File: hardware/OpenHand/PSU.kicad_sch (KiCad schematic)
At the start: 0 parts

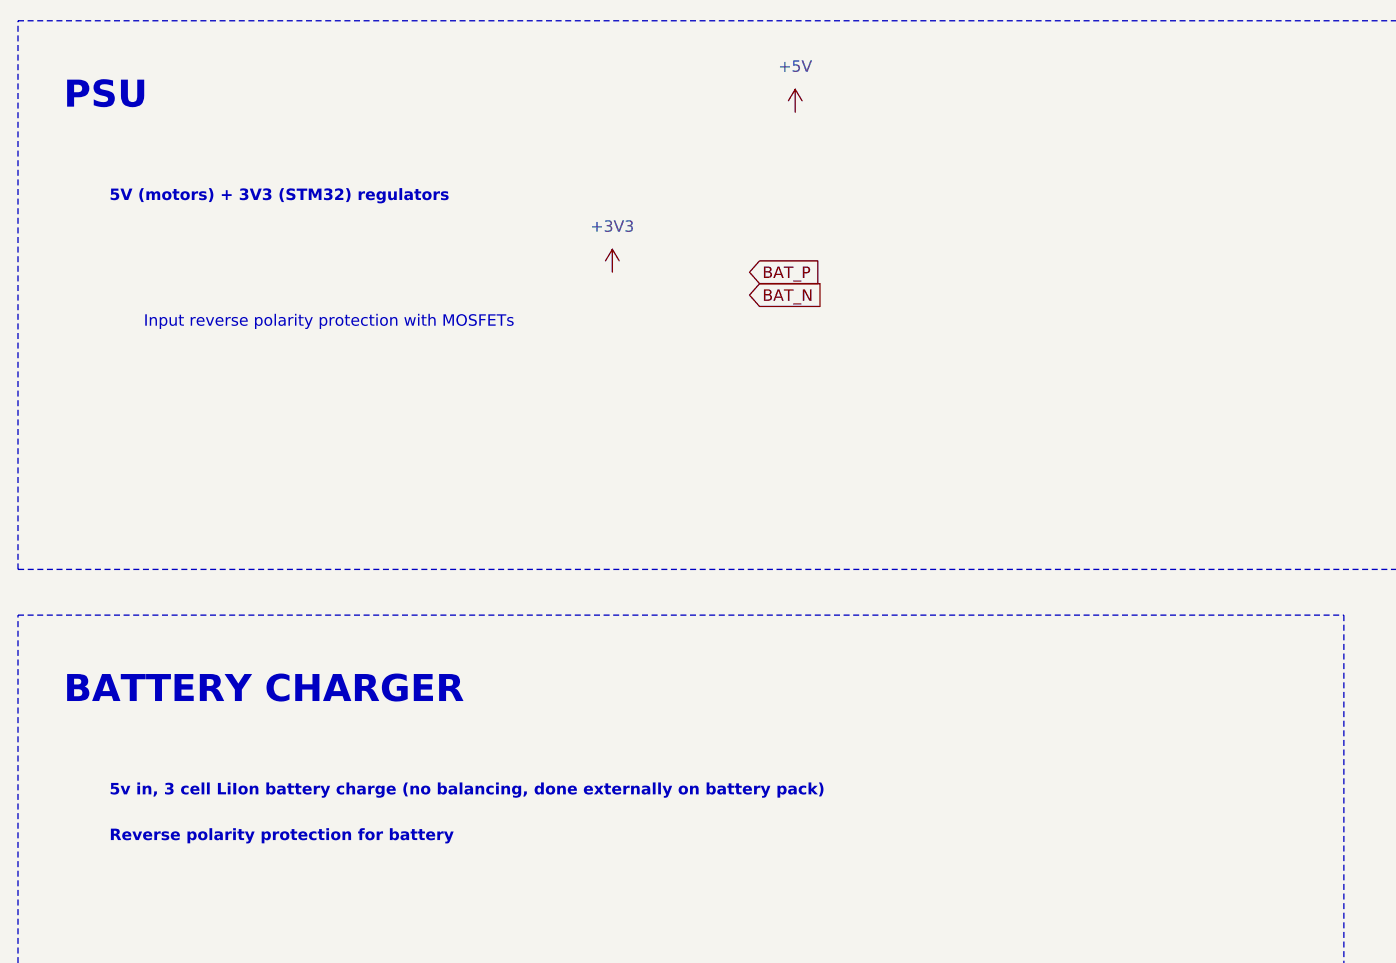
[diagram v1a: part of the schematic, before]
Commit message: Update schematic a bit
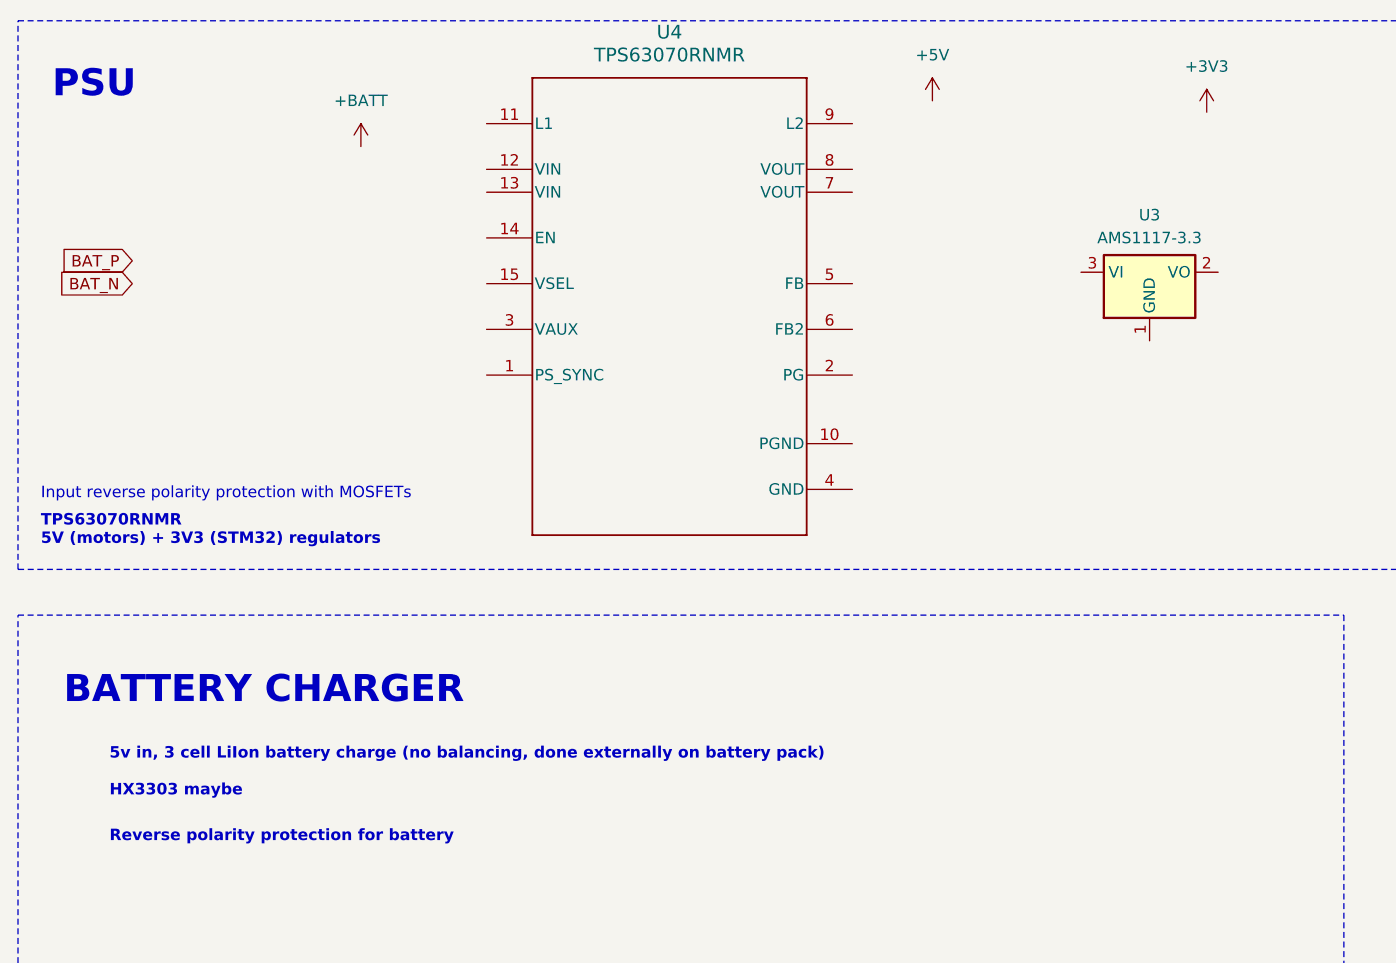
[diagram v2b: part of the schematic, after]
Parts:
- added U3: AMS1117-3.3, Package_TO_SOT_SMD:SOT-223-3_TabPin2, symbol Regulator_Linear:AMS1117-3.3
- added U4: TPS63070RNMR, symbol TPS63070RNMR:TPS63070RNMR
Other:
- note added: "5v in, 3 cell LiIon battery charge (no balancing, done externally on battery pack) HX3303 maybe"
- note added: "TPS63070RNMR 5V (motors) + 3V3 (STM32) regulators"
- note removed: "5V (motors) + 3V3 (STM32) regulators"
- note removed: "5v in, 3 cell LiIon battery charge (no balancing, done externally on battery pack)"
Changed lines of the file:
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@@
     (fill (type none))
   )
-  (text "5v in, 3 cell LiIon battery charge (no balancing, done externally on battery pack)"
+  (text "5v in, 3 cell LiIon battery charge (no balancing, done externally on battery pack)\n\nHX3303 maybe"
     (at 33.02 109.22 0)
     (effects (font (size 1.27 1.27) bold) (justify left bottom))
   )
-  (text "Input reverse polarity protection with MOSFETs" (at 36.83 57.15 0)
+  (text "Input reverse polarity protection with MOSFETs" (at 25.4 76.2 0)
     (effects (font (size 1.27 1.27)) (justify left bottom))
   )
@@
     (effects (font (size 1.27 1.27) bold) (justify left bottom))
   )
-  (text "PSU" (at 27.94 33.02 0)
+  (text "PSU" (at 26.67 31.75 0)
     (effects (font (size 3 3) (thickness 0.6) bold) (justify left bottom))
   )
@@
     (effects (font (size 3 3) (thickness 0.6) bold) (justify left bottom))
   )
-  (text "5V (motors) + 3V3 (STM32) regulators" (at 33.02 43.18 0)
+  (text "TPS63070RNMR \n5V (motors) + 3V3 (STM32) regulators"
+    (at 25.4 81.28 0)
     (effects (font (size 1.27 1.27) bold) (justify left bottom))
   )
-  (global_label "BAT_N" (shape input) (at 104.14 53.34 0) (fields_autoplaced)
-    (effects (font (size 1.27 1.27)) (justify left))
-    (property "Intersheetrefs" "${INTERSHEET_REFS}" (at 112.7495 53.34 0)
-      (effects (font (size 1.27 1.27)) (justify left) hide)
+  (global_label "BAT_N" (shape input) (at 35.56 52.07 180) (fields_autoplaced)
+    (effects (font (size 1.27 1.27)) (justify right))
+    (property "Intersheetrefs" "${INTERSHEET_REFS}" (at 26.9505 52.07 0)
+      (effects (font (size 1.27 1.27)) (justify right) hide)
     )
   )
-  (global_label "BAT_P" (shape input) (at 104.14 50.8 0) (fields_autoplaced)
-    (effects (font (size 1.27 1.27)) (justify left))
-    (property "Intersheetrefs" "${INTERSHEET_REFS}" (at 112.689 50.8 0)
-      (effects (font (size 1.27 1.27)) (justify left) hide)
+  (global_label "BAT_P" (shape input) (at 35.56 49.53 180) (fields_autoplaced)
+    (effects (font (size 1.27 1.27)) (justify right))
+    (property "Intersheetrefs" "${INTERSHEET_REFS}" (at 27.011 49.53 0)
+      (effects (font (size 1.27 1.27)) (justify right) hide)
     )
   )
-  (symbol (lib_id "power:+5V") (at 109.22 33.02 0) (unit 1)
+  (symbol (lib_id "Regulator_Linear:AMS1117-3.3") (at 148.59 50.8 0) (unit 1)
     (in_bom yes) (on_board yes) (dnp no) (fields_autoplaced)
-    (property "Reference" "#PWR01" (at 109.22 36.83 0)
+    (property "Reference" "U3" (at 148.59 44.45 0)
+      (effects (font (size 1.27 1.27)))
+    )
+    (property "Value" "AMS1117-3.3" (at 148.59 46.99 0)
+      (effects (font (size 1.27 1.27)))
+    )
+    (property "Footprint" "Package_TO_SOT_SMD:SOT-223-3_TabPin2" (at 148.59 45.72 0)
       (effects (font (size 1.27 1.27)) hide)
     )
-    (property "Value" "+5V" (at 109.22 27.94 0)
+    (property "Datasheet" "http://www.advanced-monolithic.com/pdf/ds1117.pdf" (at 151.13 57.15 0)
+      (effects (font (size 1.27 1.27)) hide)
+    )
+    (pin "1")
+    (pin "2")
+    (pin "3")
+    (instances
+      (project "OpenHand"
+        (path "/f1fbd835-8408-4592-854c-2fbec9d052ec/11b37193-b902-4bf9-977f-96c37af6f134"
+          (reference "U3") (unit 1)
+        )
+      )
+    )
+  )
+  (symbol (lib_id "power:+BATT") (at 60.96 36.83 0) (unit 1)
+    (in_bom yes) (on_board yes) (dnp no) (fields_autoplaced)
+    (property "Reference" "#PWR036" (at 60.96 40.64 0)
+      (effects (font (size 1.27 1.27)) hide)
+    )
+    (property "Value" "+BATT" (at 60.96 31.75 0)
       (effects (font (size 1.27 1.27)))
     )
-    (property "Footprint" "" (at 109.22 33.02 0)
+    (property "Footprint" "" (at 60.96 36.83 0)
       (effects (font (size 1.27 1.27)) hide)
     )
-    (property "Datasheet" "" (at 109.22 33.02 0)
+    (property "Datasheet" "" (at 60.96 36.83 0)
+      (effects (font (size 1.27 1.27)) hide)
+    )
+    (pin "1")
+    (instances
+      (project "OpenHand"
+        (path "/f1fbd835-8408-4592-854c-2fbec9d052ec/11b37193-b902-4bf9-977f-96c37af6f134"
+          (reference "#PWR036") (unit 1)
+        )
+      )
+    )
+  )
+  (symbol (lib_id "power:+5V") (at 124.46 31.75 0) (unit 1)
+    (in_bom yes) (on_board yes) (dnp no) (fields_autoplaced)
+    (property "Reference" "#PWR01" (at 124.46 35.56 0)
+      (effects (font (size 1.27 1.27)) hide)
+    )
+    (property "Value" "+5V" (at 124.46 26.67 0)
+      (effects (font (size 1.27 1.27)))
+    )
+    (property "Footprint" "" (at 124.46 31.75 0)
+      (effects (font (size 1.27 1.27)) hide)
+    )
+    (property "Datasheet" "" (at 124.46 31.75 0)
       (effects (font (size 1.27 1.27)) hide)
     )
@@
     )
   )
-  (symbol (lib_id "power:+3V3") (at 88.9 50.8 0) (unit 1)
+  (symbol (lib_id "TPS63070RNMR:TPS63070RNMR") (at 95.25 54.61 0) (unit 1)
     (in_bom yes) (on_board yes) (dnp no) (fields_autoplaced)
-    (property "Reference" "#PWR040" (at 88.9 54.61 0)
+    (property "Reference" "U4" (at 95.25 24.13 0)
+      (effects (font (size 1.524 1.524)))
+    )
+    (property "Value" "TPS63070RNMR" (at 95.25 26.67 0)
+      (effects (font (size 1.524 1.524)))
+    )
+    (property "Footprint" "" (at 95.25 54.61 0)
+      (effects (font (size 1.27 1.27) italic) hide)
+    )
+    (property "Datasheet" "TPS63070RNMR" (at 95.25 54.61 0)
+      (effects (font (size 1.27 1.27) italic) hide)
+    )
+    (pin "1")
+    (pin "10")
+    (pin "11")
+    (pin "12")
+    (pin "13")
+    (pin "14")
+    (pin "15")
+    (pin "2")
+    (pin "3")
+    (pin "4")
+    (pin "5")
+    (pin "6")
+    (pin "7")
+    (pin "8")
+    (pin "9")
+    (instances
+      (project "OpenHand"
+        (path "/f1fbd835-8408-4592-854c-2fbec9d052ec/11b37193-b902-4bf9-977f-96c37af6f134"
+          (reference "U4") (unit 1)
+        )
+      )
+    )
+  )
+  (symbol (lib_id "power:+3V3") (at 154.94 33.02 0) (unit 1)
+    (in_bom yes) (on_board yes) (dnp no) (fields_autoplaced)
+    (property "Reference" "#PWR040" (at 154.94 36.83 0)
       (effects (font (size 1.27 1.27)) hide)
     )
-    (property "Value" "+3V3" (at 88.9 45.72 0)
+    (property "Value" "+3V3" (at 154.94 27.94 0)
       (effects (font (size 1.27 1.27)))
     )
-    (property "Footprint" "" (at 88.9 50.8 0)
+    (property "Footprint" "" (at 154.94 33.02 0)
       (effects (font (size 1.27 1.27)) hide)
     )
-    (property "Datasheet" "" (at 88.9 50.8 0)
+    (property "Datasheet" "" (at 154.94 33.02 0)
       (effects (font (size 1.27 1.27)) hide)
     )

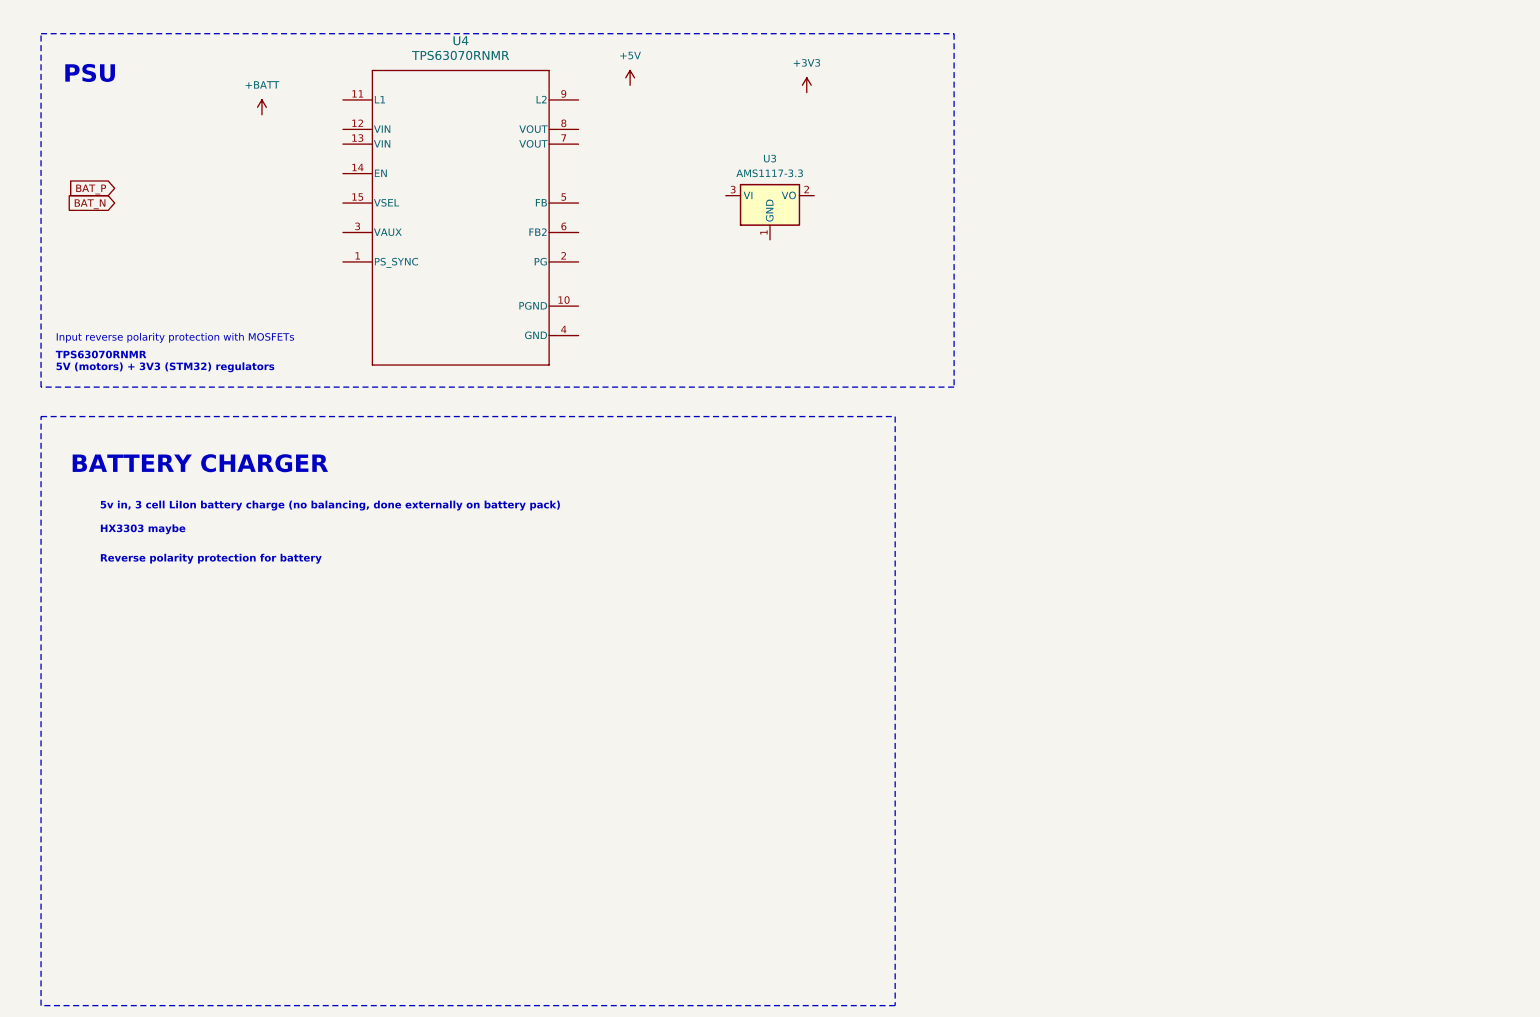
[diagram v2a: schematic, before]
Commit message: Update sch and board design
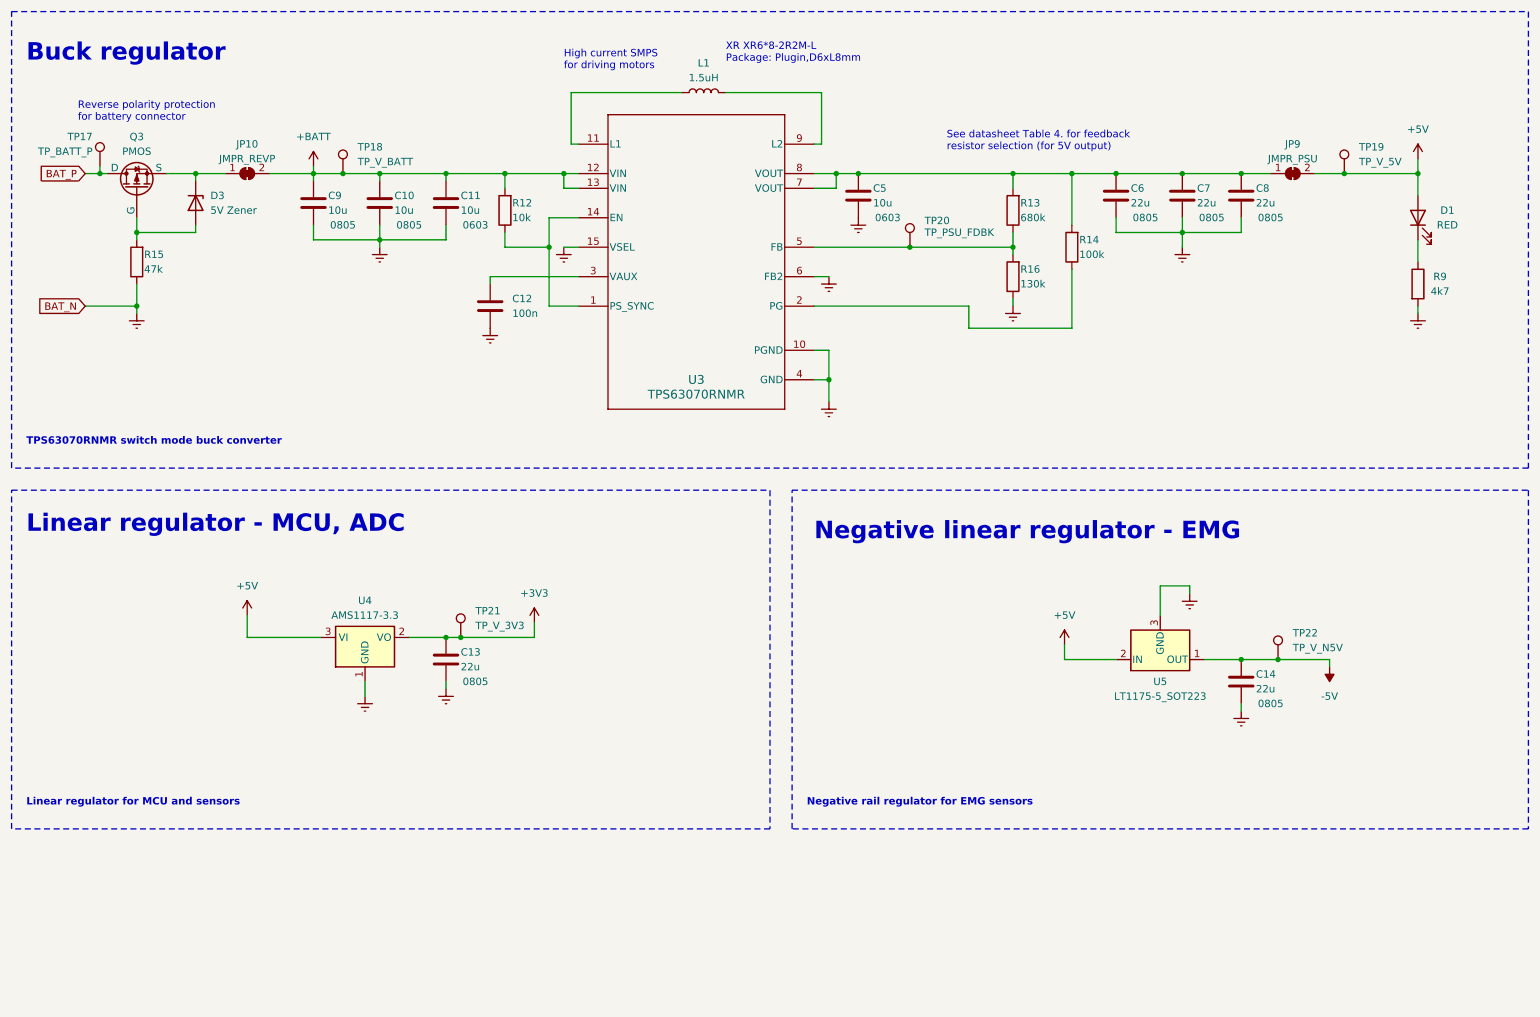
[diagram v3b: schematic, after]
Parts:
- removed U4: TPS63070RNMR, symbol TPS63070RNMR:TPS63070RNMR
- added C10, C11, C5, C9: 10u, Capacitor_SMD:C_0805_2012Metric_Pad1.18x1.45mm_HandSolder, symbol Device:C
- added C12: 100n, Capacitor_SMD:C_1206_3216Metric_Pad1.33x1.80mm_HandSolder, symbol Device:C
- added C13, C14, C6, C7, C8: 22u, Capacitor_SMD:C_0805_2012Metric_Pad1.18x1.45mm_HandSolder, symbol Device:C
- added D1: RED, LED_SMD:LED_0805_2012Metric, symbol Device:LED
- added D3: 5V Zener, Diode_THT:D_A-405_P7.62mm_Horizontal, symbol Device:D_Zener
- added JP10: JMPR_REVP, Jumper:SolderJumper-2_P1.3mm_Bridged_RoundedPad1.0x1.5mm, symbol Jumper:SolderJumper_2_Bridged
- added JP9: JMPR_PSU, Jumper:SolderJumper-2_P1.3mm_Bridged_RoundedPad1.0x1.5mm, symbol Jumper:SolderJumper_2_Bridged
- added L1: 1.5uH, Inductor_THT:L_Radial_D6.0mm_P4.00mm, symbol Device:L
- added Q3: PMOS, Package_DIP:Vishay_HVM-DIP-3_W7.62mm, symbol Simulation_SPICE:PMOS
- added R12: 10k, Resistor_SMD:R_0805_2012Metric_Pad1.20x1.40mm_HandSolder, symbol Device:R
- added R13: 680k, Resistor_SMD:R_0805_2012Metric_Pad1.20x1.40mm_HandSolder, symbol Device:R
- added R14: 100k, Resistor_SMD:R_0805_2012Metric_Pad1.20x1.40mm_HandSolder, symbol Device:R
- added R15: 47k, Resistor_SMD:R_0805_2012Metric_Pad1.20x1.40mm_HandSolder, symbol Device:R
- added R16: 130k, Resistor_SMD:R_0805_2012Metric_Pad1.20x1.40mm_HandSolder, symbol Device:R
- added R9: 4k7, Resistor_SMD:R_0805_2012Metric_Pad1.20x1.40mm_HandSolder, symbol Device:R
- added TP17: TP_BATT_P, TestPoint:TestPoint_Pad_D1.0mm, symbol Connector:TestPoint
- added TP18: TP_V_BATT, TestPoint:TestPoint_Pad_D1.0mm, symbol Connector:TestPoint
- added TP19: TP_V_5V, TestPoint:TestPoint_Pad_D1.0mm, symbol Connector:TestPoint
- added TP20: TP_PSU_FDBK, TestPoint:TestPoint_Pad_D1.0mm, symbol Connector:TestPoint
- added TP21: TP_V_3V3, TestPoint:TestPoint_Pad_D1.0mm, symbol Connector:TestPoint
- added TP22: TP_V_N5V, TestPoint:TestPoint_Pad_D1.0mm, symbol Connector:TestPoint
- added U3: TPS63070RNMR, TPS63070RNMR:TPS63070RNMR, symbol TPS63070RNMR:TPS63070RNMR
- added U5: LT1175-5_SOT223, Package_TO_SOT_SMD:SOT-223-3_TabPin2, symbol Regulator_Linear:LT1175-5_SOT223
- renumbered U3 to U4
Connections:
- net +3V3: now also U4.2 (VO), C13.1, TP21.1
- net +5V: now also U4.3 (VI), D1.2 (A), JP9.2 (B), TP19.1, U5.2 (IN)
- net +BATT: now also C10.1, C11.1, C9.1, JP10.2 (B), R12.2, TP18.1, U3.12 (VIN), U3.13 (VIN)
- net BAT_P: now also Q3.1 (D), TP17.1
- net Earth: now reaches U4.1 (GND)
- net Earth: now also C10.2, C11.2, C12.2, C13.2, C14.2, C5.2, C6.2, C7.2, C8.2, C9.2, R15.1, R16.1, R9.2, U3.10 (PGND), U3.15 (VSEL), U3.4 (GND), U3.6 (FB2), U5.3 (GND)
- new net: D3.1 (K), JP10.1 (A), Q3.3 (S)
- new net: D3.2 (A), Q3.2 (G), R15.2
- new net: R13.1, R16.2, TP20.1, U3.5 (FB)
- new net: C5.1, C6.1, C7.1, C8.1, JP9.1 (A), R13.2, R14.2, U3.7 (VOUT), U3.8 (VOUT)
- new net: D1.1 (K), R9.1
- new net: R14.1, U3.2 (PG)
- new net: C12.1, U3.3 (VAUX)
- new net: R12.1, U3.1 (PS_SYNC), U3.14 (EN)
- new net: L1.1, U3.11 (L1)
- new net: L1.2, U3.9 (L2)
- new net -5V: C14.1, TP22.1, U5.1 (OUT)
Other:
- note added: "Buck regulator"
- note added: "High current SMPS for driving motors"
- note added: "Linear regulator - MCU, ADC"
- note added: "Linear regulator for MCU and sensors"
- note added: "Negative linear regulator - EMG"
- note added: "Negative rail regulator for EMG sensors"
- note added: "Reverse polarity protection for battery connector"
- note added: "See datasheet Table 4. for feedback resistor selection (for 5V output)"
- note added: "TPS63070RNMR switch mode buck converter"
- note added: "XR XR6*8-2R2M-L Package: Plugin,D6xL8mm"
- note removed: "5v in, 3 cell LiIon battery charge (no balancing, done externally on battery pack) HX3303 maybe"
- note removed: "BATTERY CHARGER"
- note removed: "Input reverse polarity protection with MOSFETs"
- note removed: "PSU"
- note removed: "Reverse polarity protection for battery"
- note removed: "TPS63070RNMR 5V (motors) + 3V3 (STM32) regulators"
- moved on the sheet: U4
